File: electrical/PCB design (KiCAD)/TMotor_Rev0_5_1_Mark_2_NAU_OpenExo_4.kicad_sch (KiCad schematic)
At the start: 3 parts, among them J13 TFM-107-01-L-D-WT

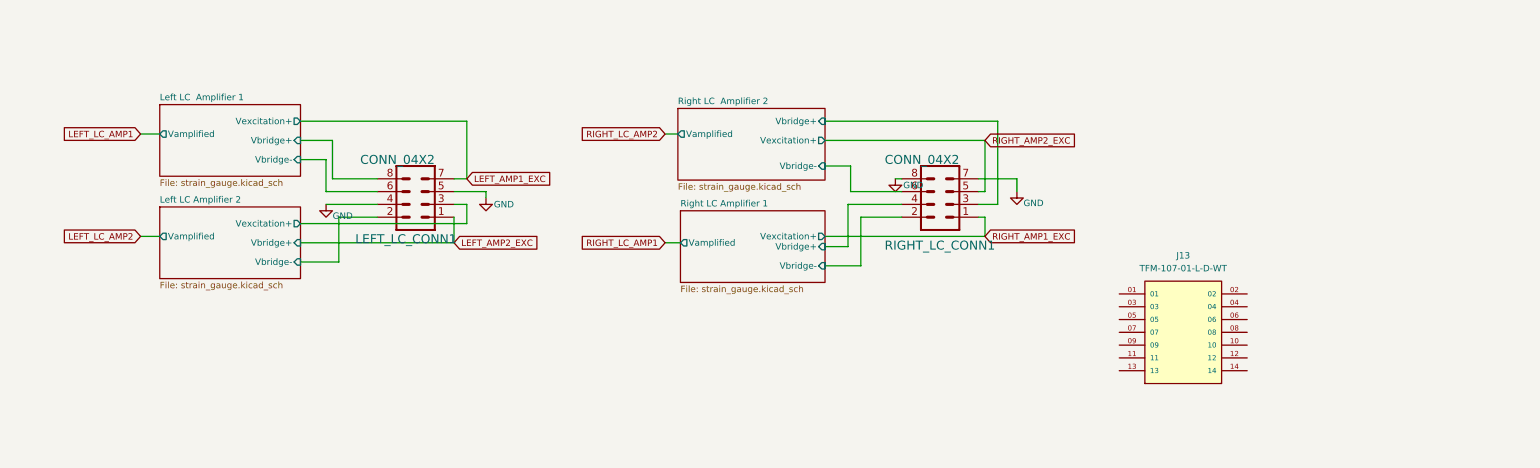
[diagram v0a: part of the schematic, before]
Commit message: PCB version v1.1.0 design+documentation
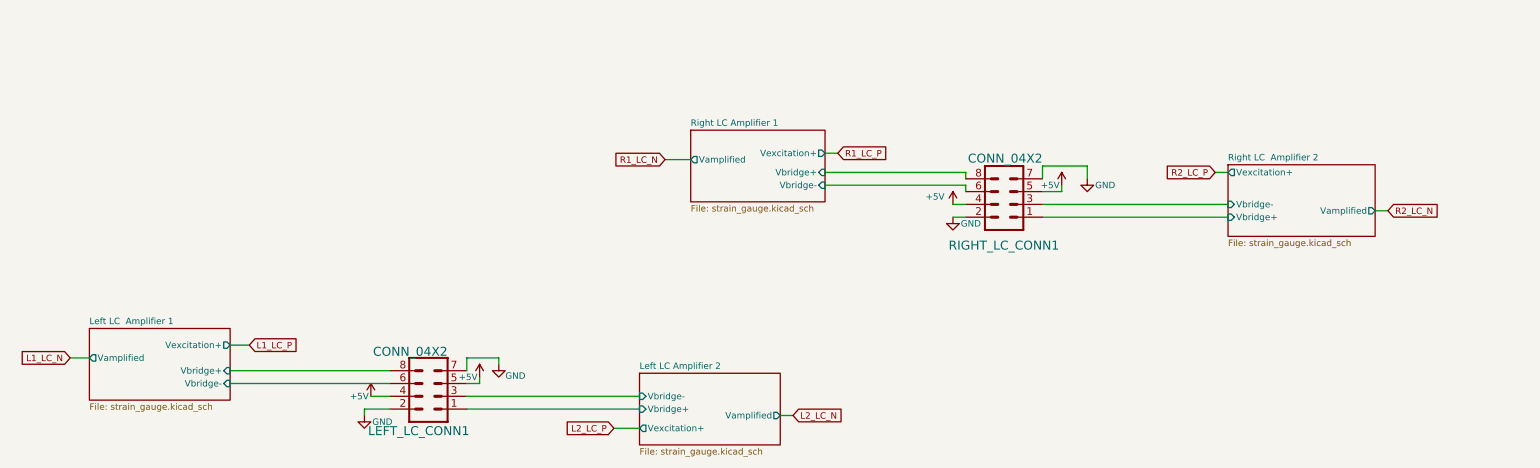
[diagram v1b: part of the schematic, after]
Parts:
- removed J13: TFM-107-01-L-D-WT, ISDF connector:SAMTEC_TFM-107-01-L-D-WT, symbol TFM-107-01-L-D-WT:TFM-107-01-L-D-WT
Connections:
- net LEFT_AMP1_EXC is gone; now on net GND: LEFT_LC_CONN1.7
- net Left LC Amplifier 2/Vexcitation+ is gone; now on net Left LC Amplifier 2/Vbridge-: LEFT_LC_CONN1.3
- net RIGHT_AMP1_EXC is gone; now on net Right LC  Amplifier 2/Vbridge+: RIGHT_LC_CONN1.1
- net GND: now also LEFT_LC_CONN1.2, RIGHT_LC_CONN1.2; no longer LEFT_LC_CONN1.4, LEFT_LC_CONN1.5, RIGHT_LC_CONN1.8
- net Left LC Amplifier 2/Vbridge-: no longer LEFT_LC_CONN1.2
- net Right LC  Amplifier 2/Vbridge+: no longer RIGHT_LC_CONN1.3
- net Right LC  Amplifier 2/Vbridge-: now also RIGHT_LC_CONN1.3; no longer RIGHT_LC_CONN1.6
- net Right LC Amplifier 1/Vbridge+: now also RIGHT_LC_CONN1.8; no longer RIGHT_LC_CONN1.4
- net Right LC Amplifier 1/Vbridge-: now also RIGHT_LC_CONN1.6; no longer RIGHT_LC_CONN1.2
- net LEFT_AMP2_EXC renamed Left LC Amplifier 2/Vbridge+
- net RIGHT_AMP2_EXC renamed +5V
- net +5V: now also LEFT_LC_CONN1.4, LEFT_LC_CONN1.5, RIGHT_LC_CONN1.4
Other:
- moved on the sheet: LEFT_LC_CONN1, RIGHT_LC_CONN1
